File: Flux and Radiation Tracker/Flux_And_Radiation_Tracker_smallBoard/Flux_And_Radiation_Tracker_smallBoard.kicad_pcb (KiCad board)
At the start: 2 copper layers, 36.5 x 32 mm, 12 parts, among them J1 Conn_01x07, U2 MMC5983MA

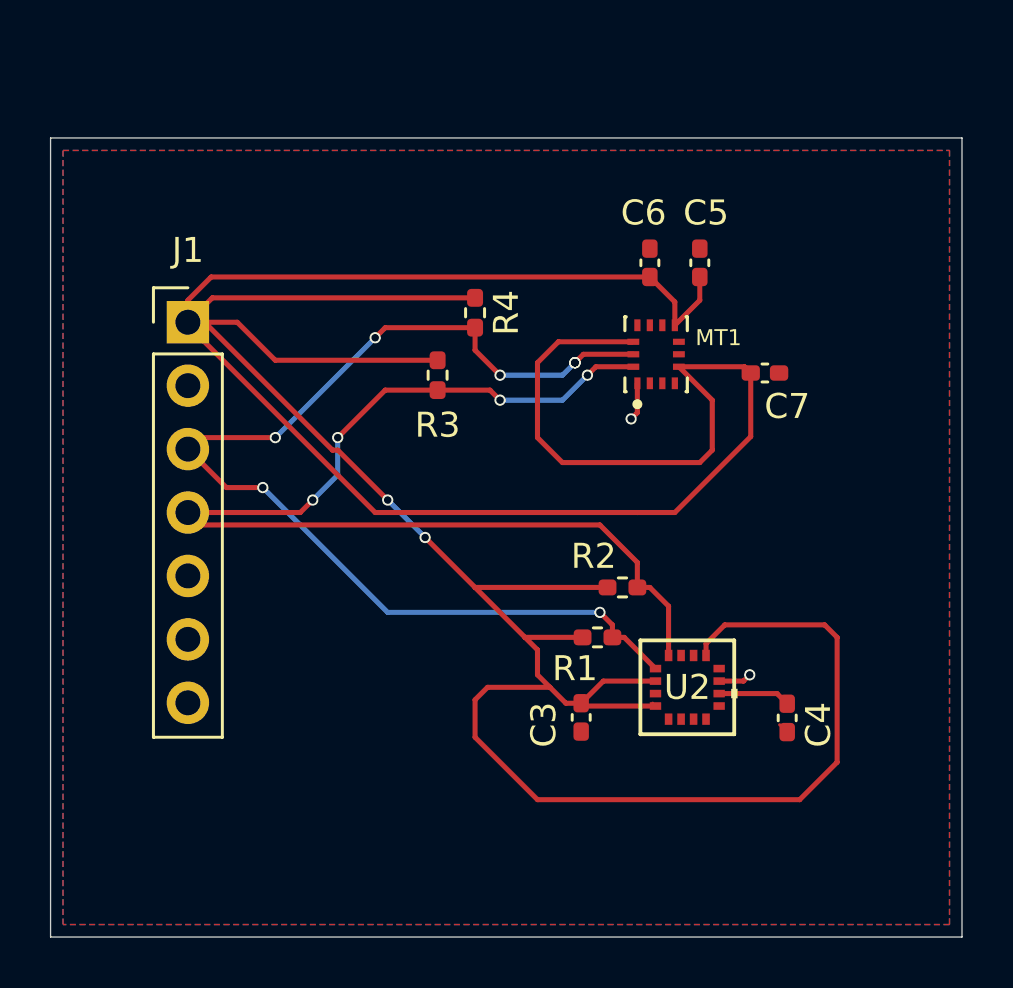
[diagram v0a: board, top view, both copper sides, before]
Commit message: Add files via upload
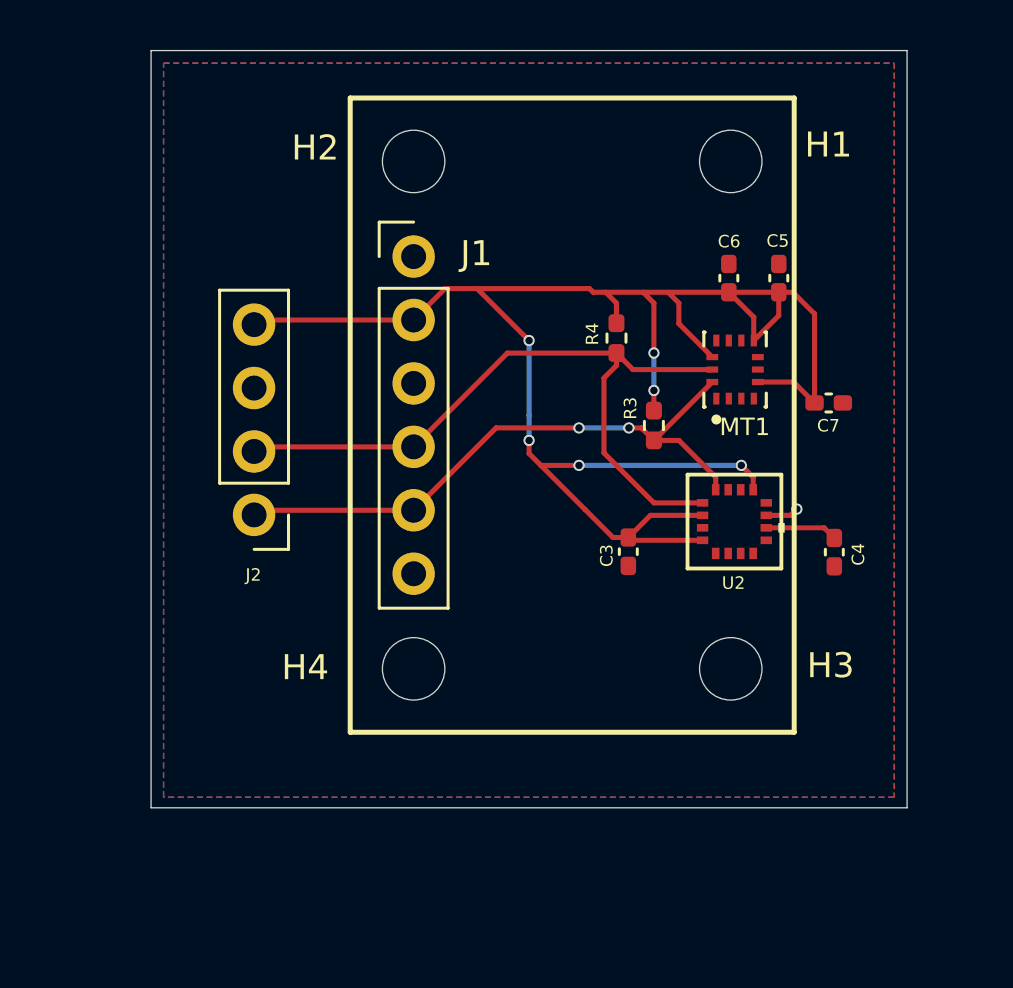
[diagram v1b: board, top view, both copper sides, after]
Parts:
- removed R1, R2: 2.7k, Resistor_SMD:R_0402_1005Metric_Pad0.72x0.64mm_HandSolder
- added H1: MountingHole, MountingHole:MountingHole_2.5mm, F.Cu at (157.2, 80.4)
- added H2: MountingHole, MountingHole:MountingHole_2.5mm, F.Cu at (144.5, 80.4)
- added H3: MountingHole, MountingHole:MountingHole_2.5mm, F.Cu at (157.2, 100.8)
- added H4: MountingHole, MountingHole:MountingHole_2.5mm, F.Cu at (144.5, 100.8)
- added J2: Conn_01x04_Pin, Connector_PinHeader_2.54mm:PinHeader_1x04_P2.54mm_Vertical, F.Cu at (138.2, 94.6)
- J1: value Conn_01x07 -> Conn_01x06_Pin; footprint Connector_PinHeader_2.54mm:PinHeader_1x07_P2.54mm_Vertical -> Connector_PinHeader_2.54mm:PinHeader_1x06_P2.54mm_Vertical
- moved J1 9.41 mm to (144.5, 84.2)
- moved R3 8.89 mm to (154.2, 91.0)
- moved C3 6.90 mm to (153.1, 96.1)
- moved C4 6.90 mm to (161.4, 96.1)
- moved U2 6.90 mm to (157.4, 94.9)
- moved R4 5.75 mm to (152.7, 87.5)
- moved MT1 3.22 mm to (157.4, 88.8)
- moved C5 3.22 mm to (159.2, 85.1)
- moved C6 3.22 mm to (157.2, 85.1)
- moved C7 2.82 mm to (161.2, 90.1)
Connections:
- J1 pad 1: +3.3V -> unconnected-(J1-Pin_1-Pad1)
- J1 pad 2: GND -> +3.3V
- J1 pad 3: I2C_SCL -> GND
- J1 pad 4: I2C_SDA -> I2C_SCL
- J1 pad 5: unconnected-(J1-Pin_5-Pad5) -> I2C_SDA
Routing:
- net +3.3V: track 168.0 -> 72.4 mm, vias 2 -> 6
- net I2C_SDA: track 44.8 -> 24.6 mm, vias 4 -> 2
- net I2C_SCL: track 44.2 -> 29.2 mm, vias 8 -> 0
- net GND: track 2.89 -> 1.33 mm, vias 2 -> 1
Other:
- board size 36.5 x 32 mm -> 30.3 x 30.3 mm
